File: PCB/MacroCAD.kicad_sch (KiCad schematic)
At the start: 26 parts, among them J1 Conn_01x04, SW1 SW_Push, SW10 SW_Push, SW11 SW_Push, SW12 SW_Push, SW2 SW_Push, SW3 SW_Push, SW4 SW_Push, SW5 SW_Push, SW6 SW_Push, SW7 SW_Push, SW8 SW_Push, SW9 SW_Push, U1 MOUDLE-SEEEDUINO-XIAO

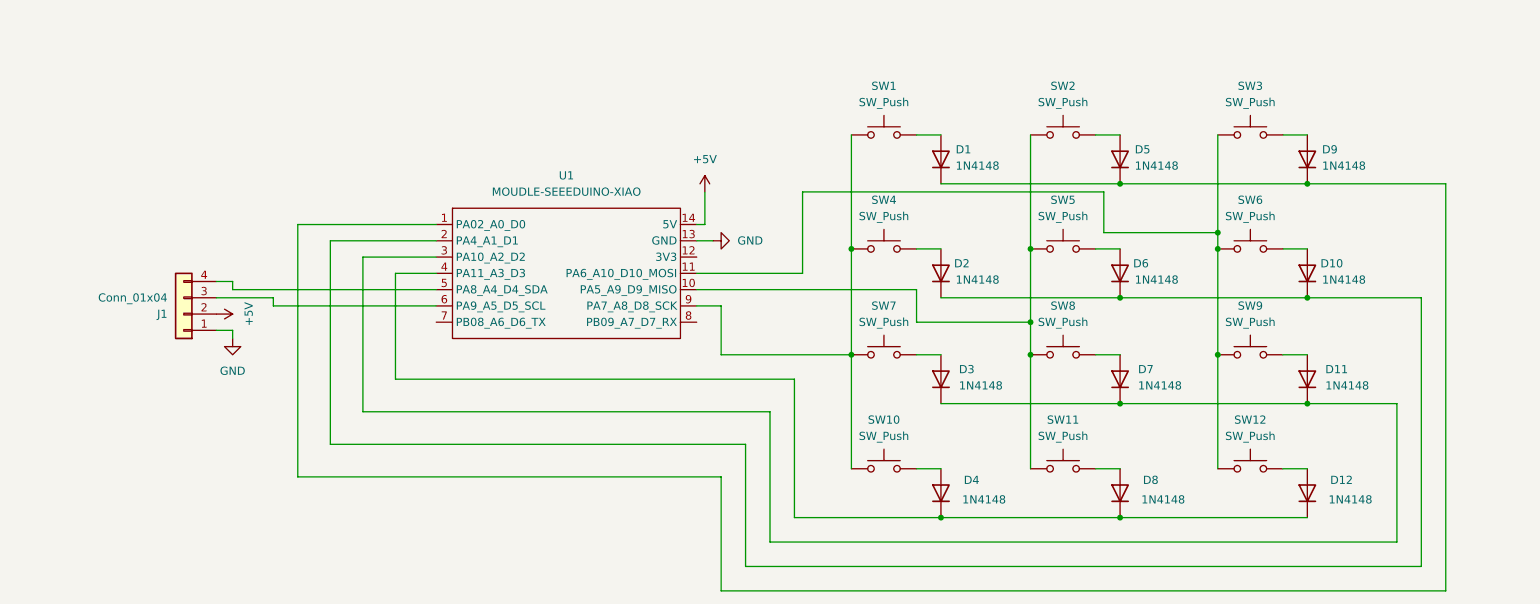
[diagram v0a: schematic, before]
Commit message: PCB's final toutch
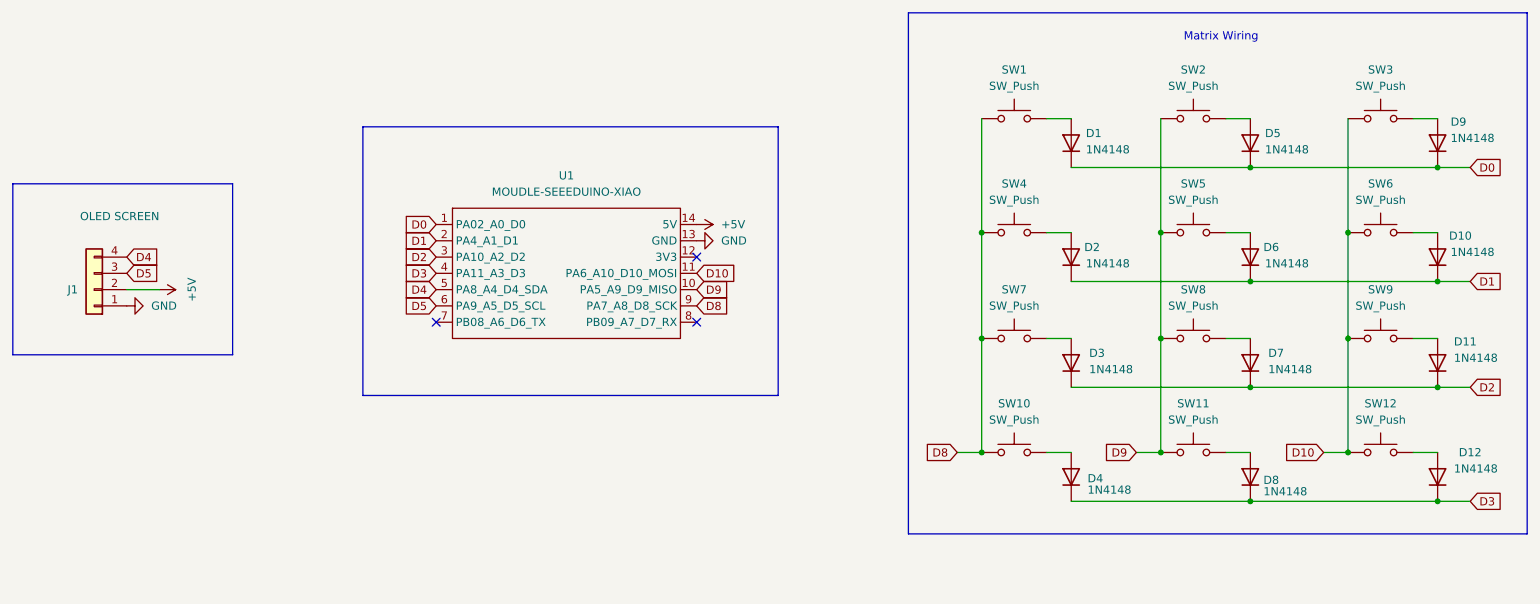
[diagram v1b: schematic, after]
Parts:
- J1: value Conn_01x04 -> OLED SCREEN
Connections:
- net D8: now reaches SW1.1, SW10.1, SW4.1, SW7.1, U1.9 (PA7_A8_D8_SCK)
- net D3: now reaches D12.1 (K), D4.1 (K), D8.1 (K), U1.4 (PA11_A3_D3)
- net D9: now reaches SW11.1, SW2.1, SW5.1, SW8.1, U1.10 (PA5_A9_D9_MISO)
- net D10: now reaches SW12.1, SW3.1, SW6.1, SW9.1, U1.11 (PA6_A10_D10_MOSI)
- net D0: now reaches D1.1 (K), D5.1 (K), D9.1 (K), U1.1 (PA02_A0_D0)
- net D1: now reaches D10.1 (K), D2.1 (K), D6.1 (K), U1.2 (PA4_A1_D1)
- net D2: now reaches D11.1 (K), D3.1 (K), D7.1 (K), U1.3 (PA10_A2_D2)
- net D4: now reaches J1.4 (Pin_4), U1.5 (PA8_A4_D4_SDA)
- net D5: now reaches J1.3 (Pin_3), U1.6 (PA9_A5_D5_SCL)
- no-connect marks 0 -> 3
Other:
- note added: "Matrix Wiring"
- moved on the sheet: D1, D10, D11, D12, D2, D3, D4, D5, D6, D7, D8, D9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
